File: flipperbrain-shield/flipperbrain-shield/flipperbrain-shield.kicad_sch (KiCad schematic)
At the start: 6 parts, among them J1 Power, J2 Digital/PWM, J3 Analog, J4 Digital/PWM

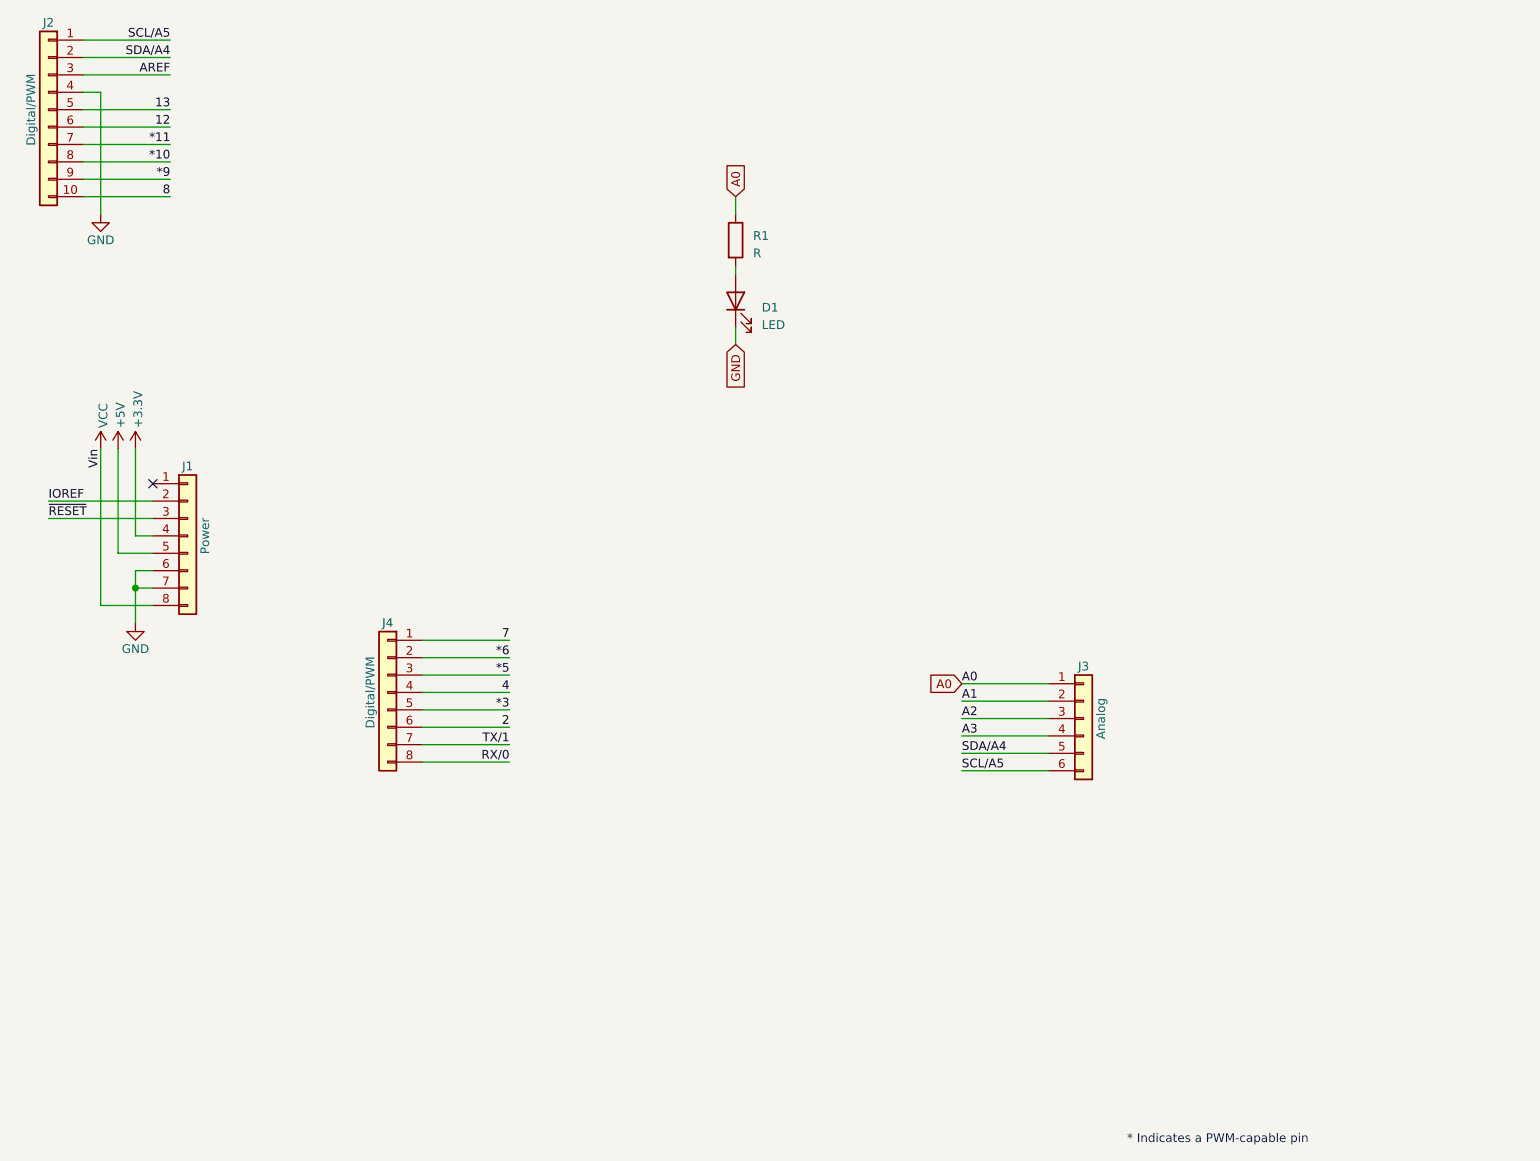
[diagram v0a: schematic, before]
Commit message: nc
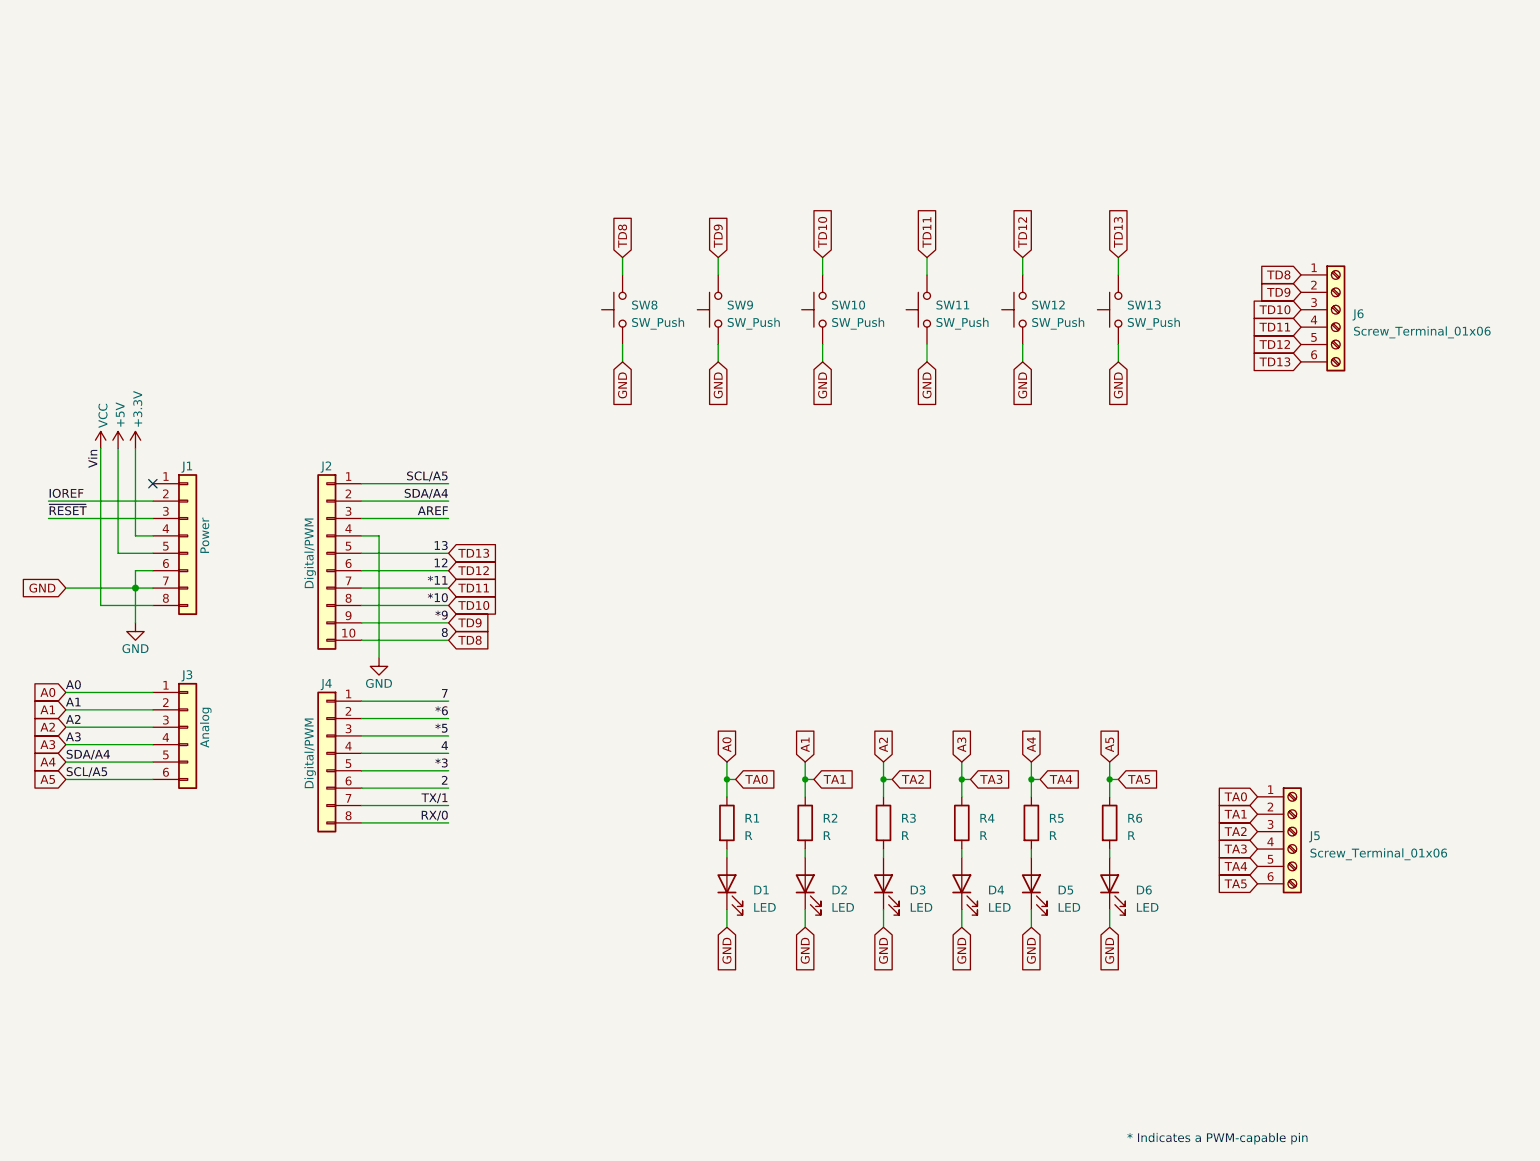
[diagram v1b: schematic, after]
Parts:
- added D2, D3, D4, D5, D6: LED, LED_THT:LED_D5.0mm, symbol Device:LED
- added J5, J6: Screw_Terminal_01x06, TerminalBlock_Phoenix:TerminalBlock_Phoenix_PT-1,5-6-3.5-H_1x06_P3.50mm_Horizontal, symbol Connector:Screw_Terminal_01x06
- added R2, R3, R4, R5, R6: R, Resistor_THT:R_Axial_DIN0207_L6.3mm_D2.5mm_P10.16mm_Horizontal, symbol Device:R
- added SW10, SW11, SW12, SW13, SW8, SW9: SW_Push, Button_Switch_THT:SW_PUSH_6mm, symbol Switch:SW_Push
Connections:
- net A0: now also J5.1 (Pin_1)
- net A1: now also J5.2 (Pin_2), R2.1
- net A2: now also J5.3 (Pin_3), R3.1
- net A3: now also J5.4 (Pin_4), R4.1
- net GND: now also D2.1 (K), D3.1 (K), D4.1 (K), D5.1 (K), D6.1 (K), SW10.1, SW11.1, SW12.1, SW13.1, SW8.1, SW9.1
- net *10 renamed TD10
- net TD10: now also J6.3 (Pin_3), SW10.2
- net *11 renamed TD11
- net TD11: now also J6.4 (Pin_4), SW11.2
- net *9 renamed TD9
- net TD9: now also J6.2 (Pin_2), SW9.2
- net 12 renamed TD12
- net TD12: now also J6.5 (Pin_5), SW12.2
- net 13 renamed TD13
- net TD13: now also J6.6 (Pin_6), SW13.2
- net 8 renamed TD8
- net TD8: now also J6.1 (Pin_1), SW8.2
- net SCL/A5 renamed A5
- net A5: now also J5.6 (Pin_6), R6.1
- net SDA/A4 renamed A4
- net A4: now also J5.5 (Pin_5), R5.1
- new net: D5.2 (A), R5.2
- new net: D3.2 (A), R3.2
- new net: D4.2 (A), R4.2
- new net: D6.2 (A), R6.2
- new net: D2.2 (A), R2.2
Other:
- moved on the sheet: D1, J2, J3, J4, R1

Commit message: nc
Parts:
- J5, J6: footprint TerminalBlock_Phoenix:TerminalBlock_Phoenix_PT-1,5-6-3.5-H_1x06_P3.50mm_Horizontal -> TerminalBlock_Phoenix:TerminalBlock_Phoenix_MPT-0,5-6-2.54_1x06_P2.54mm_Horizontal
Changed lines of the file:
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@@
       (effects (font (size 1.27 1.27)) (justify left))
     )
-    (property "Footprint" "TerminalBlock_Phoenix:TerminalBlock_Phoenix_PT-1,5-6-3.5-H_1x06_P3.50mm_Horizontal" (at 201.93 134.62 0)
+    (property "Footprint" "TerminalBlock_Phoenix:TerminalBlock_Phoenix_MPT-0,5-6-2.54_1x06_P2.54mm_Horizontal" (at 201.93 134.62 0)
       (effects (font (size 1.27 1.27)) hide)
     )
@@
       (effects (font (size 1.27 1.27)) (justify left))
     )
-    (property "Footprint" "TerminalBlock_Phoenix:TerminalBlock_Phoenix_PT-1,5-6-3.5-H_1x06_P3.50mm_Horizontal" (at 208.28 58.42 0)
-      (effects (font (size 1.27 1.27)) hide)
-    )
+    (property "Footprint" "TerminalBlock_Phoenix:TerminalBlock_Phoenix_MPT-0,5-6-2.54_1x06_P2.54mm_Horizontal" (at 208.28 58.42 0)
+      (effects (font (size 1.27 1.27)) hide)
+    )
